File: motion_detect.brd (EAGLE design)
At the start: 60 x 52 mm, 82 parts, among them CON1 PINHEAD_1X02-2.54, CON2 PINHEAD_1X01-2.54, CON3 PINHEAD_1X08-2.54, CON4 PINHEAD_1X05-2.54, CON5 PINHEAD_1X01-2.54, CON6 USB-2, IC1 5.0, IC2 LTC4054, IC3 3.3, IC4 ATMEGA168-TQFP32, J1 POWER_JACKPTH, Q1 IRLML2502-SOT23, Q2 IRLML2244TRPBF, Q3 IRLML2502-SOT23, Q4 IRLML2502-SOT23, SW1 TACT_SWITCH

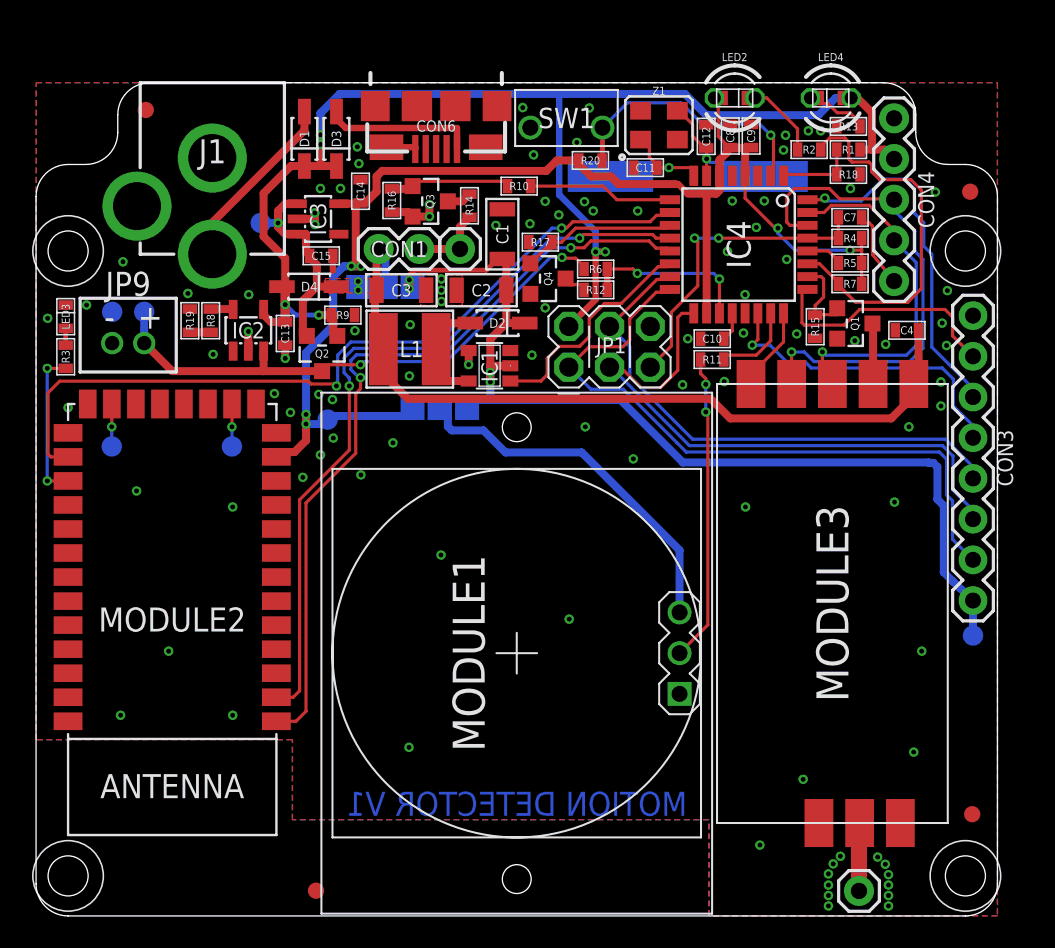
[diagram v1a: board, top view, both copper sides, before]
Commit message: new version
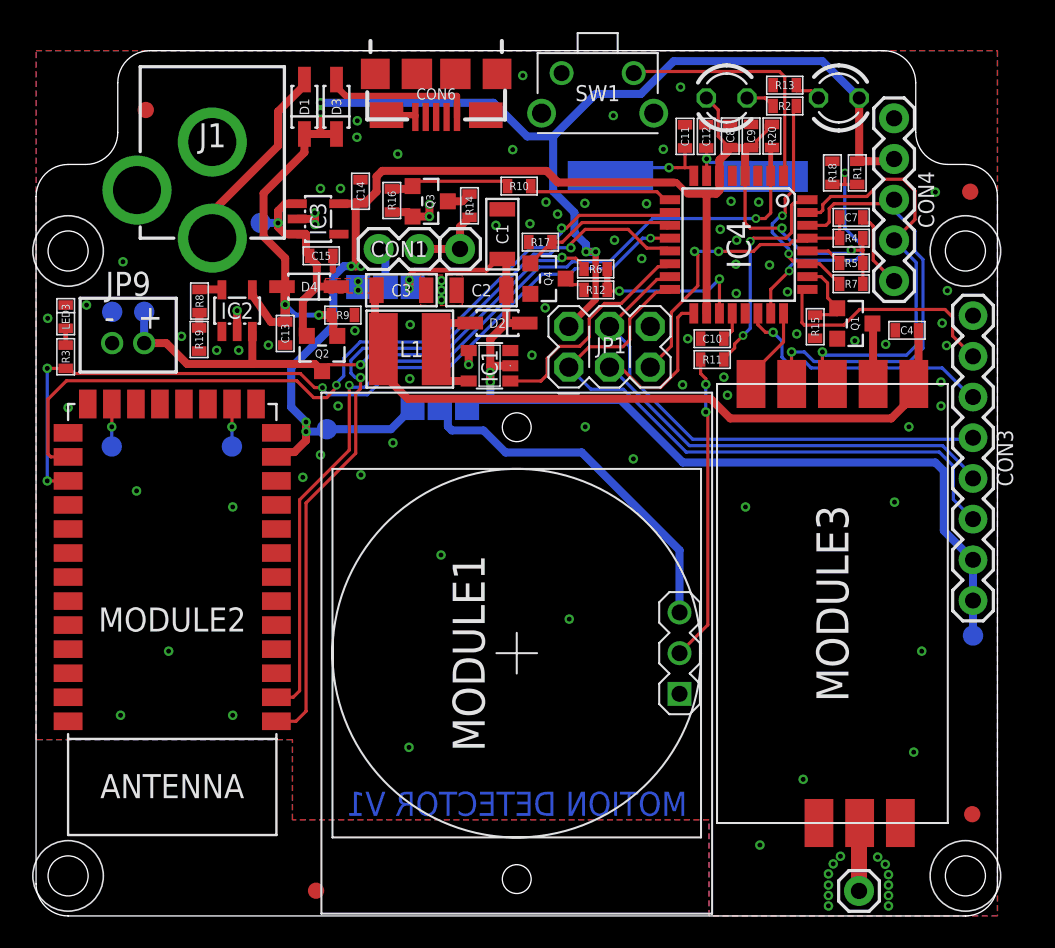
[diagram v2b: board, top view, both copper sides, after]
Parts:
- removed LED2, LED4: LED-0603, rc:LED0603
- removed Z1: 8MHz, led_matrix_master_lib:OSCILLATOR-3.2X2.5
- SW1: value TACT_SWITCH -> TACT_SWITCH-TC-206; device motion_detect_masterlib:IT-1102V -> motion_detect_masterlib:TC-0206
- moved R20 11.4 mm to (15.9, 22.7), turned to 270 degrees
- moved R13 4.74 mm to (16.7, 25.9)
- moved C11 3.15 mm to (10.5, 22.6), turned to 90 degrees
- moved R2 3.12 mm to (16.7, 24.6)
- moved SW1 2.49 mm to (5.05, 25.4), turned to 180 degrees
- moved CON6 2.00 mm to (-5.03, 25.3)
- moved D1 2.00 mm to (-13.2, 24.5)
- moved D3 2.00 mm to (-11.2, 24.5)
- moved R1 1.55 mm to (21.2, 20.4), turned to 270 degrees
- moved IC2 1.41 mm to (-17.4, 11.8)
- moved R8 1.41 mm to (-19.8, 12.4)
- moved R19 1.31 mm to (-19.8, 9.97), turned to 270 degrees
- moved R18 1.00 mm to (19.7, 20.4), turned to 90 degrees
- moved J1 1.00 mm to (-19.0, 30.0)
- moved TP6 0.60 mm to (-11.8, 4.38)
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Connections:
- removed net CHRG_LED: IC2.1
- removed net N$19: MODULE2.24, R3.2
- net A0: now also R1.2, R18.1; no longer R11.1
- net A7: now also CON3.6; no longer CON3.5
- net D2: now also R11.1; no longer CON3.6
- net D3: now also SW1.1; no longer R1.2, R18.1
- net D4: now also MODULE2.2; no longer SW1.P$2
- net D8: now also MODULE2.24, R3.2; no longer MODULE2.2
- net GND: now also SW1.2; no longer SW1.P$1
- net MISO: now also CON3.3; no longer CON3.2
- net MOSI: now also CON3.5; no longer CON3.4
- net N$12: no longer LED4.C
- net N$2: no longer LED2.C
- net N$6: no longer Z1.3
- net N$8: no longer Z1.1
- net SCK: now also CON3.4; no longer CON3.3
- net SUP: no longer LED4.A
- net VDD_3V3: no longer LED2.A
- net VDD_5V: now also CON3.2
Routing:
- net D4: track 16.7 -> 57.5 mm, vias 1 -> 2
- net D3: track 4.91 -> 15.9 mm
- net A0: track 5.38 -> 16.0 mm, vias 0 -> 2
- net N$19: track 9.63 -> 0.00 mm, vias 2 -> 0
- net A4: track 23.7 -> 14.7 mm, vias 0 -> 2
- net D2: track 22.2 -> 13.7 mm, vias 1 -> 2
- net D8: track 47.4 -> 53.0 mm, vias 2 -> 4
- net TXO: track 23.2 -> 27.6 mm
- net VDD_3V3: track 88.2 -> 91.9 mm
- net RXI: track 31.0 -> 27.4 mm
- net N$2: track 5.30 -> 1.84 mm
- net A7: track 19.7 -> 16.6 mm
- net N$6: track 9.06 -> 5.97 mm
- net MISO: track 42.1 -> 39.6 mm
- net SCK: track 37.8 -> 35.3 mm
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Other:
- board size 60 x 52 mm -> 60 x 54 mm
